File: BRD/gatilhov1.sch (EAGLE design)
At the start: 38 parts, among them IC1 TINY13-20SSU, IC2 LD117AS28TR, Q1 IRL7843, T1 BC817, T2 BC807, T3 BC817

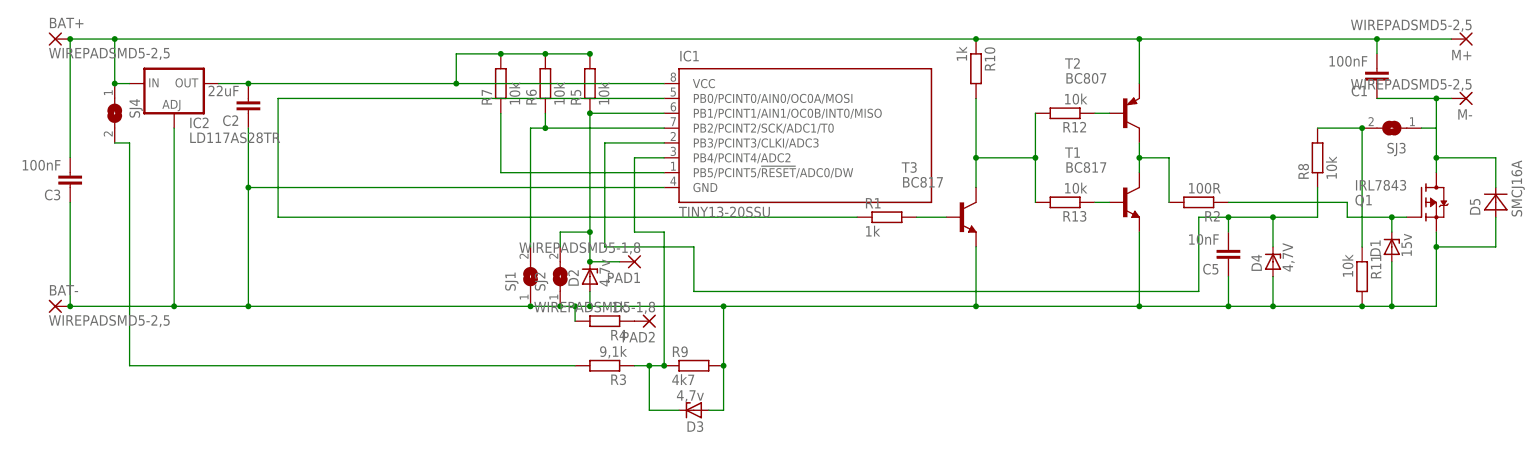
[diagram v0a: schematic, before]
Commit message: Signed-off-by: Jéfferson Pimenta Melo <jefferson.pimenta@hotmail.com>
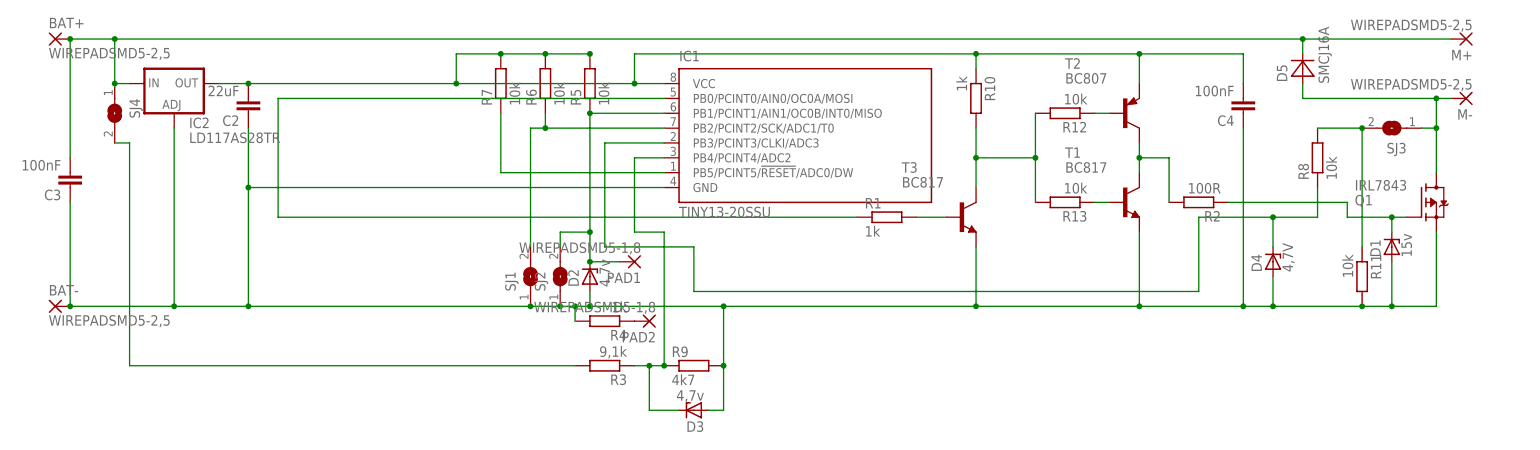
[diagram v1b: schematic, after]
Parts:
- removed C1: 100nF, rcl:C-EUC0805K
- removed C5: 10nF, rcl:C-EUC0805K
- added C4: 100nF, rcl:C-EUC1206K
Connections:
- removed net N$3: C2.2, IC1.VCC, IC2.OUT, R5.2, R6.2, R7.2
- new net N$20: C2.2, C4.2, IC1.VCC, IC2.OUT, R10.1, R5.2, R6.2, R7.2, T2.E
- net N$1: now also C4.1; no longer C5.1, D5.A
- net N$14: now also D5.C; no longer C1.2, R10.1, T2.E
- net N$2: now also D5.A; no longer C1.1, D5.C
- net N$5: no longer C5.2
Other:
- moved on the sheet: D5, R10
